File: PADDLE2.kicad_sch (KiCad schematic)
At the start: 0 parts

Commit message: R20260915
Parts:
- added C11, C12: .1, symbol Device:C
- added R19: R, symbol Device:R_US
- added R20: 470, symbol Device:R_US
- added R21: 56K, symbol Device:R_US
- added RV1: R_Potentiometer_US, symbol Device:R_Potentiometer_US
- added UA7: 7420, Package_DIP:DIP-14_W7.62mm_Socket_LongPads, symbol 74xx_IEEE:7420
- added UA8: 7493, Package_DIP:DIP-14_W7.62mm_Socket_LongPads, symbol 74xx_IEEE:7493
- added UA9: NE555P, Package_DIP:DIP-8_W7.62mm_Socket_LongPads, symbol Timer:NE555P
- added UB7, UG3: 7400, Package_DIP:DIP-14_W7.62mm_Socket_LongPads, symbol 74xx:7400
- added UC9: 7404, Package_DIP:DIP-14_W7.62mm_Socket_LongPads, symbol 74xx_IEEE:7404
- added UG2: 7427, Package_DIP:DIP-14_W7.62mm_Socket_LongPads, symbol 74xx_IEEE:7427
- added UH3: 74LS74, Package_DIP:DIP-14_W7.62mm_Socket_LongPads, symbol 74xx:74LS74
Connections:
- new net: C12.1, R20.1
- new net: R20.2, UA9.5 (CONT)
- new net: R19.1, UH3.1 (~{R})
- new net: C11.1, R21.2, UA9.6 (THRES), UA9.7 (DISCH)
- new net: UG2.13, UG2.9, UG3.8
- new net: UA7.1, UA8.1 (~{CKB}), UA8.12 (Q0)
- new net: UA7.2, UA8.9 (Q1)
- new net: UA7.4, UA8.8 (Q2)
- new net: UA7.5, UA8.11 (Q3)
- new net: UA7.6, UB7.12, UB7.9
- new net: UA8.14 (~{CKA}), UB7.8
- new net: UA8.2 (R0(1)), UA8.3 (R0(2)), UA9.3 (OUT), UC9.1
- new net: UB7.13, UC9.2
- new net: UG3.9, UH3.6 (~{Q})
- new net: R21.1, RV1.2, RV1.3
- new net +3.3V: UA7.14 (VCC), UA8.5 (VCC), UC9.14 (VCC), UG2.14 (VCC), UG2.14 (VCC)
- new net +5V: R19.2, RV1.1, UA9.4 (~{RST}), UA9.8 (VCC)
- new net 128H: UG3.10, UH3.2 (D)
- new net 256H: UG2.10
- new net 4H: UH3.3 (C)
- new net GND: C11.2, C12.2, UA7.7 (GND), UA8.10 (GND), UA9.1 (GND), UC9.7 (GND), UG2.7 (GND), UG2.7 (GND)
- new net PAD1: UG2.8
- new net PAD2: UG2.12
- new net /256H: UG2.2
- new net /256V: UA9.2 (TRIG)
- new net /ATTRACT: UH3.4 (~{S})
- new net /HSYNC: UB7.10
- new net /VPAD1: UG2.11
- new net /VPAD2: UB7.11, UG2.1
- no-connect marks 0 -> 1
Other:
- company: (none) -> Atari
- title: (none) -> PONG

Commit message: R20260918
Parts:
- UA7, UA8, UB7, UC9, UG2, UG3, UH3: footprint Package_DIP:DIP-14_W7.62mm_Socket_LongPads -> pong:pong_DIP-14_W7.62mm_Socket_LongPads
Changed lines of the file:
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@@
 			)
 		)
-		(property "Footprint" "Package_DIP:DIP-14_W7.62mm_Socket_LongPads"
+		(property "Footprint" "pong:pong_DIP-14_W7.62mm_Socket_LongPads"
 			(at 115.57 173.99 0)
 			(hide yes)
@@
 			)
 		)
-		(property "Footprint" "Package_DIP:DIP-14_W7.62mm_Socket_LongPads"
+		(property "Footprint" "pong:pong_DIP-14_W7.62mm_Socket_LongPads"
 			(at 241.3 80.01 0)
 			(hide yes)
@@
 			)
 		)
-		(property "Footprint" "Package_DIP:DIP-14_W7.62mm_Socket_LongPads"
+		(property "Footprint" "pong:pong_DIP-14_W7.62mm_Socket_LongPads"
 			(at 154.94 72.39 0)
 			(hide yes)
@@
 			)
 		)
-		(property "Footprint" "Package_DIP:DIP-14_W7.62mm_Socket_LongPads"
+		(property "Footprint" "pong:pong_DIP-14_W7.62mm_Socket_LongPads"
 			(at 124.46 34.29 0)
 			(hide yes)
@@
 			)
 		)
-		(property "Footprint" "Package_DIP:DIP-14_W7.62mm_Socket_LongPads"
+		(property "Footprint" "pong:pong_DIP-14_W7.62mm_Socket_LongPads"
 			(at 115.57 133.35 0)
 			(hide yes)
@@
 			)
 		)
-		(property "Footprint" "Package_DIP:DIP-14_W7.62mm_Socket_LongPads"
+		(property "Footprint" "pong:pong_DIP-14_W7.62mm_Socket_LongPads"
 			(at 45.72 120.65 0)
 			(hide yes)
@@
 			)
 		)
-		(property "Footprint" "Package_DIP:DIP-14_W7.62mm_Socket_LongPads"
+		(property "Footprint" "pong:pong_DIP-14_W7.62mm_Socket_LongPads"
 			(at 182.88 72.39 0)
 			(hide yes)
@@
 			)
 		)
-		(property "Footprint" "Package_DIP:DIP-14_W7.62mm_Socket_LongPads"
+		(property "Footprint" "pong:pong_DIP-14_W7.62mm_Socket_LongPads"
 			(at 72.39 125.73 0)
 			(hide yes)
@@
 			)
 		)
-		(property "Footprint" "Package_DIP:DIP-14_W7.62mm_Socket_LongPads"
+		(property "Footprint" "pong:pong_DIP-14_W7.62mm_Socket_LongPads"
 			(at 154.94 44.45 0)
 			(hide yes)

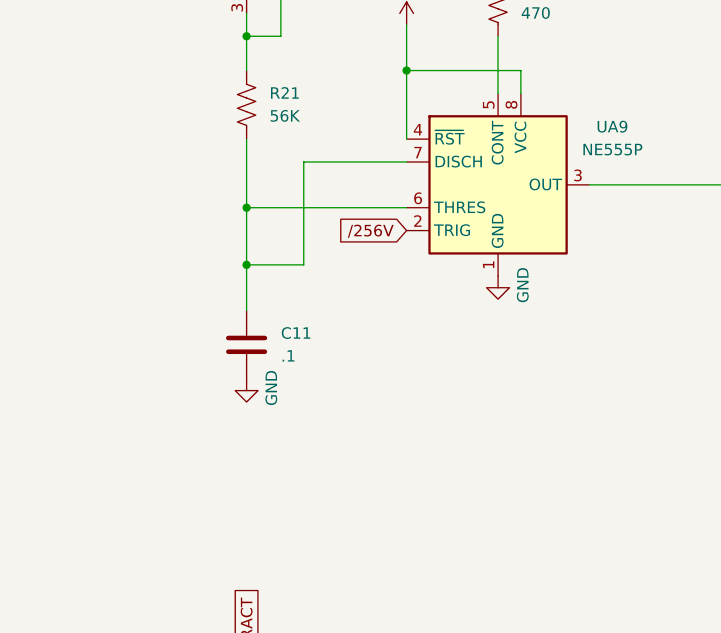
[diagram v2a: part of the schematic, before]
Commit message: R20260922
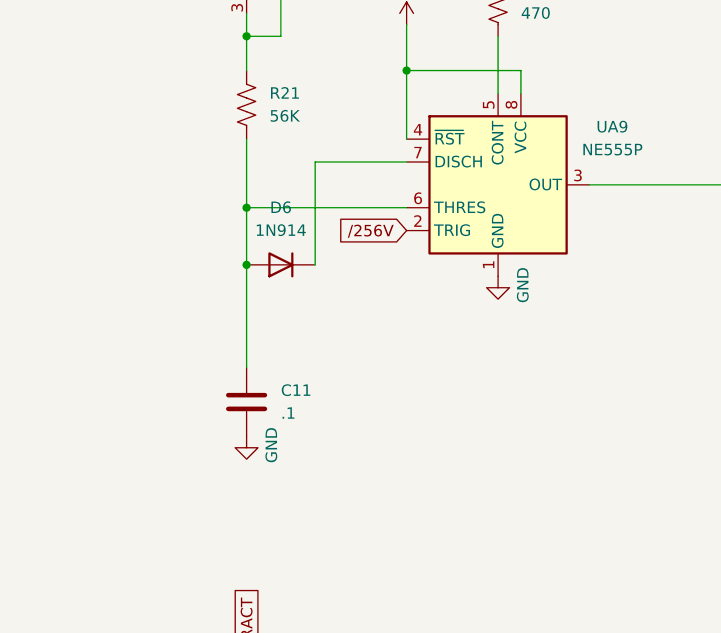
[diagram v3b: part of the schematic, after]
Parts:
- added D6: 1N914, Diode_THT:D_DO-35_SOD27_P10.16mm_Horizontal, symbol Diode:1N914
- C11, C12: footprint (none) -> Capacitor_THT:C_Axial_L3.8mm_D2.6mm_P10.00mm_Horizontal
- R19, R20, R21: footprint (none) -> Resistor_THT:R_Axial_DIN0207_L6.3mm_D2.5mm_P10.16mm_Horizontal
- RV1: footprint (none) -> Potentiometer_THT:Potentiometer_Bourns_3296Y_Vertical
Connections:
- net at C11.1, R21.2, UA9.6 (THRES): now also D6.2 (A); no longer UA9.7 (DISCH)
- new net: D6.1 (K), UA9.7 (DISCH)
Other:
- moved on the sheet: C11
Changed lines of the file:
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@@
 	(wire
 		(pts
-			(xy 45.72 66.04) (xy 45.72 71.12)
+			(xy 45.72 66.04) (xy 45.72 77.47)
 		)
 		(stroke
@@
 	(wire
 		(pts
-			(xy 52.07 54.61) (xy 52.07 66.04)
+			(xy 53.34 54.61) (xy 53.34 66.04)
 		)
 		(stroke
@@
 	(wire
 		(pts
-			(xy 63.5 54.61) (xy 52.07 54.61)
+			(xy 63.5 54.61) (xy 53.34 54.61)
 		)
 		(stroke
@@
 		)
 	)
-	(wire
-		(pts
-			(xy 52.07 66.04) (xy 45.72 66.04)
-		)
-		(stroke
-			(width 0)
-			(type default)
-		)
-	)
 	(global_label "{slash}HSYNC"
 		(shape input)
@@
 			)
 		)
-		(property "Footprint" ""
+		(property "Footprint" "Resistor_THT:R_Axial_DIN0207_L6.3mm_D2.5mm_P10.16mm_Horizontal"
 			(at 74.676 37.084 90)
 			(hide yes)
@@
 			)
 		)
-		(property "Footprint" ""
+		(property "Footprint" "Resistor_THT:R_Axial_DIN0207_L6.3mm_D2.5mm_P10.16mm_Horizontal"
 			(at 46.736 142.494 90)
 			(hide yes)
@@
 	(symbol
 		(lib_id "Device:C")
-		(at 45.72 74.93 0)
+		(at 45.72 81.28 0)
 		(unit 1)
 		(body_style 1)
@@
 		(fields_autoplaced yes)
 		(property "Reference" "C11"
-			(at 49.53 73.6599 0)
+			(at 49.53 80.0099 0)
 			(show_name no)
 			(do_not_autoplace no)
@@
 		)
 		(property "Value" ".1"
-			(at 49.53 76.1999 0)
+			(at 49.53 82.5499 0)
 			(show_name no)
 			(do_not_autoplace no)
@@
 			)
 		)
-		(property "Footprint" ""
-			(at 46.6852 78.74 0)
+		(property "Footprint" "Capacitor_THT:C_Axial_L3.8mm_D2.6mm_P10.00mm_Horizontal"
+			(at 46.6852 85.09 0)
 			(hide yes)
 			(show_name no)
@@
 		)
 		(property "Datasheet" ""
-			(at 45.72 74.93 0)
+			(at 45.72 81.28 0)
 			(hide yes)
 			(show_name no)
@@
 		)
 		(property "Description" "Unpolarized capacitor"
-			(at 45.72 74.93 0)
+			(at 45.72 81.28 0)
 			(hide yes)
 			(show_name no)
@@
 			)
 		)
-		(property "Footprint" ""
+		(property "Footprint" "Capacitor_THT:C_Axial_L3.8mm_D2.6mm_P10.00mm_Horizontal"
 			(at 87.3252 33.02 0)
 			(hide yes)
@@
 	)
 	(symbol
+		(lib_id "Diode:1N914")
+		(at 49.53 66.04 180)
+		(unit 1)
+		(body_style 1)
+		(exclude_from_sim no)
+		(in_bom yes)
+		(on_board yes)
+		(in_pos_files yes)
+		(dnp no)
+		(fields_autoplaced yes)
+		(property "Reference" "D6"
+			(at 49.53 59.69 0)
+			(show_name no)
+			(do_not_autoplace no)
+			(effects
+				(font
+					(size 1.27 1.27)
+				)
+			)
+		)
+		(property "Value" "1N914"
+			(at 49.53 62.23 0)
+			(show_name no)
+			(do_not_autoplace no)
+			(effects
+				(font
+					(size 1.27 1.27)
+				)
+			)
+		)
+		(property "Footprint" "Diode_THT:D_DO-35_SOD27_P10.16mm_Horizontal"
+			(at 49.53 61.595 0)
+			(hide yes)
+			(show_name no)
+			(do_not_autoplace no)
+			(effects
+				(font
+					(size 1.27 1.27)
+				)
+			)
+		)
+		(property "Datasheet" "http://www.vishay.com/docs/85622/1n914.pdf"
+			(at 49.53 66.04 0)
+			(hide yes)
+			(show_name no)
+			(do_not_autoplace no)
+			(effects
+				(font
+					(size 1.27 1.27)
+				)
+			)
+		)
+		(property "Description" "100V 0.3A Small Signal Fast Switching Diode, DO-35"
+			(at 49.53 66.04 0)
+			(hide yes)
+			(show_name no)
+			(do_not_autoplace no)
+			(effects
+				(font
+					(size 1.27 1.27)
+				)
+			)
+		)
+		(property "Sim.Device" "D"
+			(at 49.53 66.04 0)
+			(hide yes)
+			(show_name no)
+			(do_not_autoplace no)
+			(effects
+				(font
+					(size 1.27 1.27)
+				)
+			)
+		)
+		(property "Sim.Pins" "1=K 2=A"
+			(at 49.53 66.04 0)
+			(hide yes)
+			(show_name no)
+			(do_not_autoplace no)
+			(effects
+				(font
+					(size 1.27 1.27)
+				)
+			)
+		)
+		(pin "2"
+		)
+		(pin "1"
+		)
+		(instances
+			(project "pong"
+				(path "/6c55baa6-be38-444e-ac95-9cecf812b759/1d942afb-67a3-4399-a8e9-cfe14f4ae65e"
+					(reference "D6")
+					(unit 1)
+				)
+			)
+		)
+	)
+	(symbol
 		(lib_id "74xx_IEEE:7420")
 		(at 241.3 80.01 0)
@@
 	(symbol
 		(lib_id "power:GND")
-		(at 45.72 78.74 0)
+		(at 45.72 85.09 0)
 		(unit 1)
 		(body_style 1)
@@
 		(dnp no)
 		(property "Reference" "#PWR075"
-			(at 45.72 85.09 0)
+			(at 45.72 91.44 0)
 			(hide yes)
 			(show_name no)
@@
 		)
 		(property "Value" "GND"
-			(at 48.514 77.724 90)
+			(at 48.514 84.074 90)
 			(show_name no)
 			(do_not_autoplace no)
@@
 		)
 		(property "Footprint" ""
-			(at 45.72 78.74 0)
+			(at 45.72 85.09 0)
 			(hide yes)
 			(show_name no)
@@
 		)
 		(property "Datasheet" ""
-			(at 45.72 78.74 0)
+			(at 45.72 85.09 0)
 			(hide yes)
 			(show_name no)
@@
 		)
 		(property "Description" "Power symbol creates a global label with name \"GND\" , ground"
-			(at 45.72 78.74 0)
+			(at 45.72 85.09 0)
 			(hide yes)
 			(show_name no)
@@
 			)
 		)
-		(property "Footprint" ""
+		(property "Footprint" "Potentiometer_THT:Potentiometer_Bourns_3296Y_Vertical"
 			(at 45.72 34.29 0)
 			(hide yes)
@@
 			)
 		)
-		(property "Footprint" ""
+		(property "Footprint" "Resistor_THT:R_Axial_DIN0207_L6.3mm_D2.5mm_P10.16mm_Horizontal"
 			(at 46.736 48.514 90)
 			(hide yes)
